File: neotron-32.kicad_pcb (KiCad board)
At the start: 2 copper layers, 166.9 x 140.7 mm, 97 parts, among them J1 Conn_02x06, J10 micro SD Card, J11 Conn_02x13_Top_Bottom, J12 AVR-ISP-6, J13 DE9 Male, J14 DE9 Male, J15 Double-mini-DIN-6, J17 DB15HD_Female, J18 Conn_02x05, J2 Conn_02x06, J3 Conn_02x04, J4 DIN-5 180 degree, J5 DIN-5 180 degree, J7 3.5mm Audio Jack TRS, J8 Conn_01x03_Male, J9 USB_B, SW1 SW_Push_DPDT_ON_OFF, SW2 SW_Push_DPDT_ON_MO, U1 TM4C123G_Launchpad, U2 74LS14, U3 6N138, U4 TC1262-33, U5 MCP23S17_SP, U6 ATmega328-PU, U7 MCP7940N-xP, U8 ICL3232CPZMAX, Y1 32,768 Hz

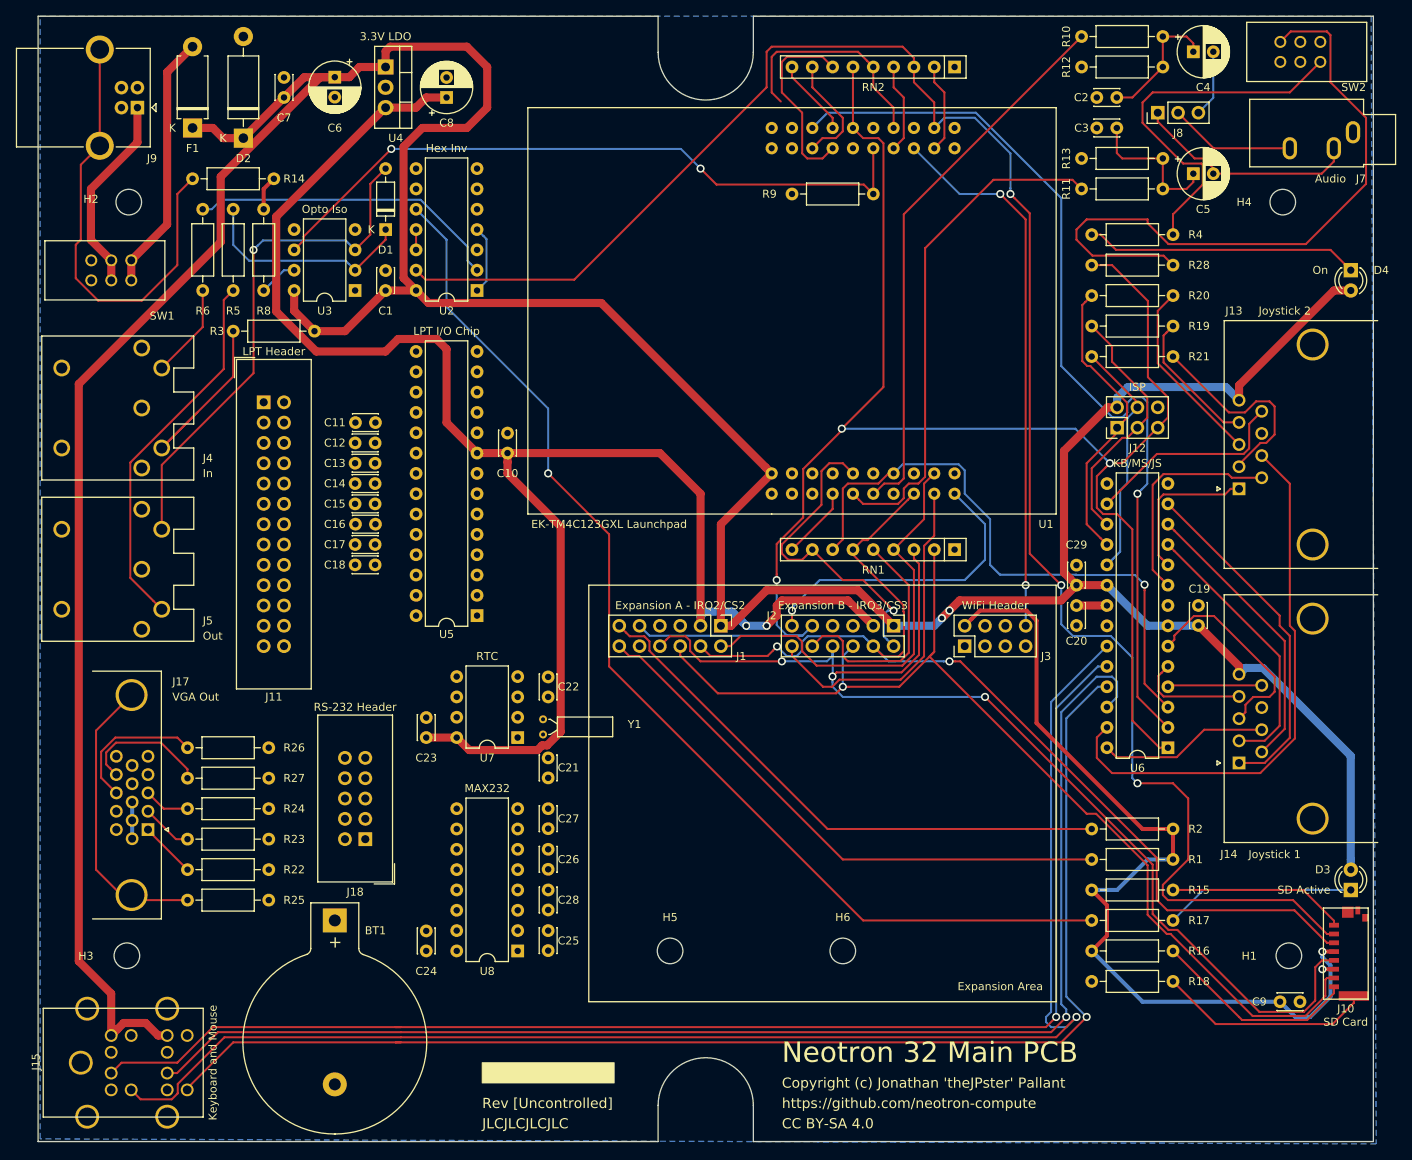
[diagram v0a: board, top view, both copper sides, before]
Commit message: More tracking.
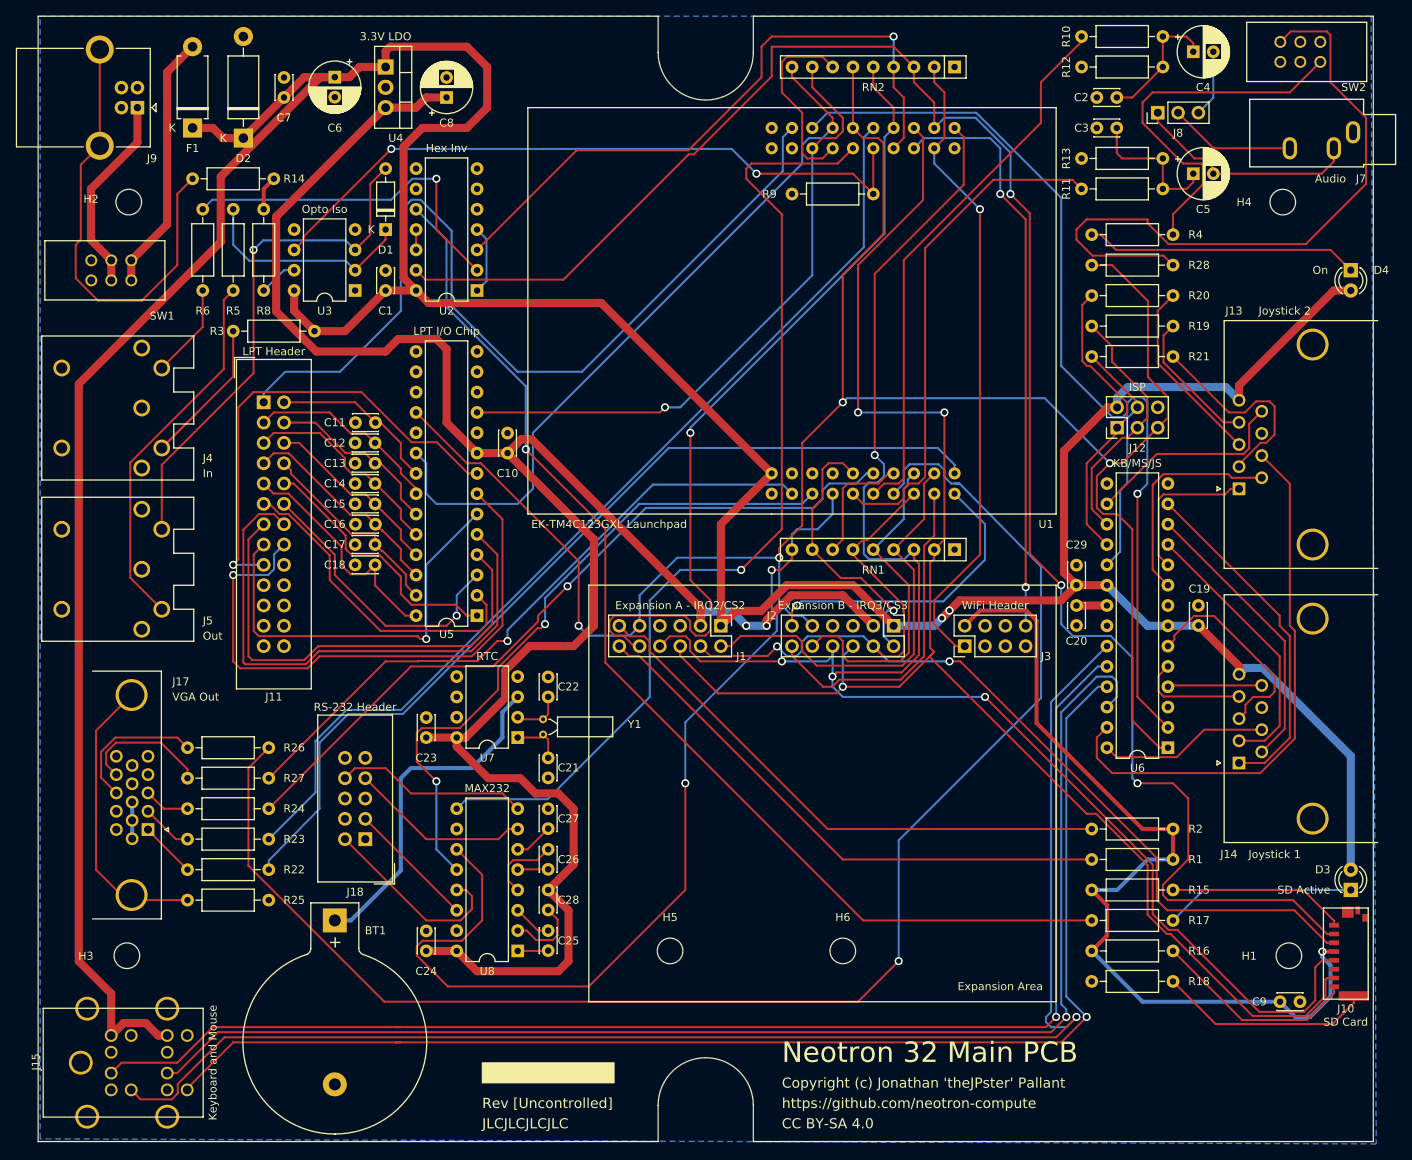
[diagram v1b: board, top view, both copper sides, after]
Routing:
- net /PB4_VGA_HSYNC: track 0.00 -> 190.3 mm, vias 0 -> 1
- net /PB7_VGA_GREEN: track 0.00 -> 124.2 mm
- net /PC5_U1CTS: track 0.00 -> 123.5 mm, vias 0 -> 1
- net /PF1_VGA_RED: track 0.00 -> 115.0 mm
- net /~PB2_STROBE: track 0.00 -> 114.0 mm
- net /PB1_U1TX: track 9.09 -> 120.9 mm, vias 0 -> 2
- net /PD3_VGA_BLUE: track 0.00 -> 94.0 mm, vias 0 -> 1
- net /PB0_U1RX: track 0.00 -> 84.5 mm, vias 0 -> 2
- net /~PF0_IRQ1: track 9.72 -> 92.2 mm
- net /PB5_VGA_VSYNC: track 0.00 -> 81.9 mm, vias 0 -> 1
- net /~PB6_SPI_CS2: track 28.5 -> 103.7 mm, vias 0 -> 1
- net /Parallel Printer/RESET: track 0.00 -> 73.8 mm, vias 0 -> 1
- net /Parallel Printer/~LF: track 0.00 -> 69.3 mm
- net /PD7_U2TX: track 11.2 -> 80.4 mm, vias 0 -> 1
- net /PC7_MIDI_OUT: track 11.2 -> 80.4 mm, vias 0 -> 1
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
